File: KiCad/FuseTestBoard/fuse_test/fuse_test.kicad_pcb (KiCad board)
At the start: 2 copper layers, 20.2 x 16 mm, 1 part

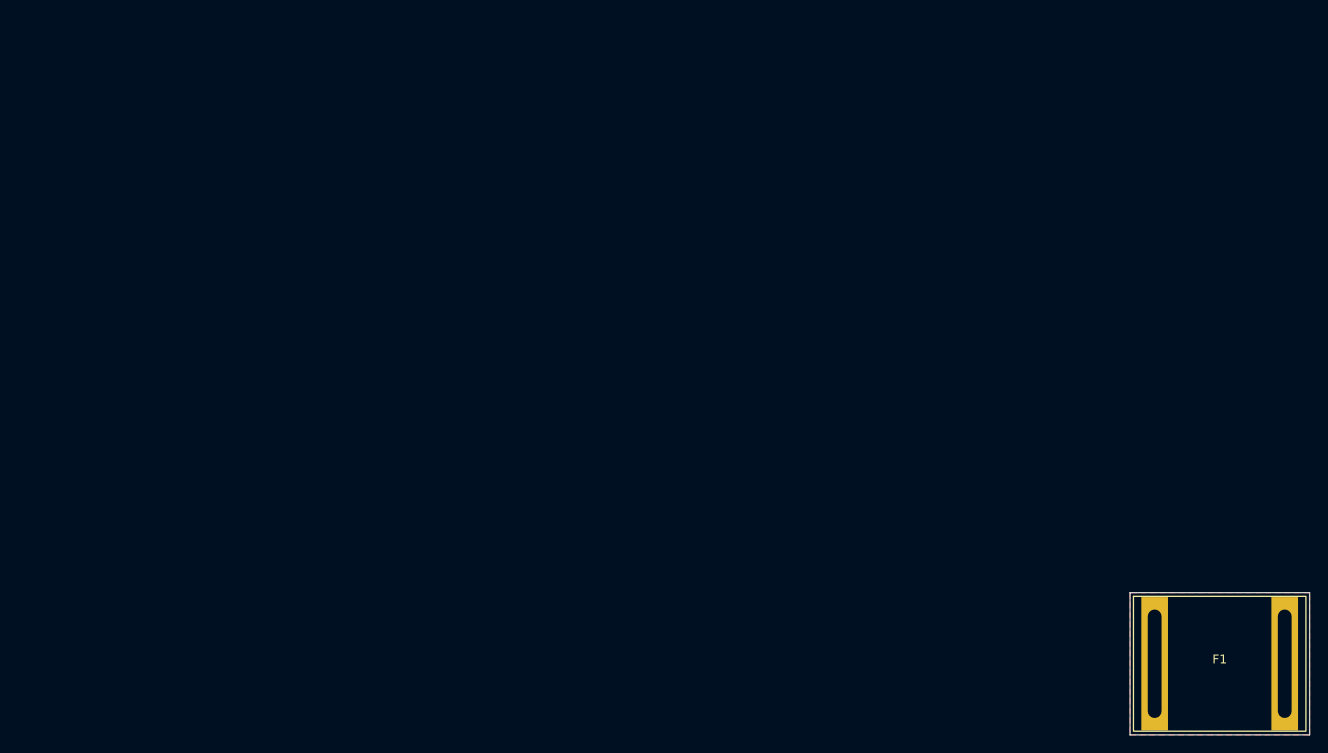
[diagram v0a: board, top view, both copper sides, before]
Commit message: adjustments to main board revision
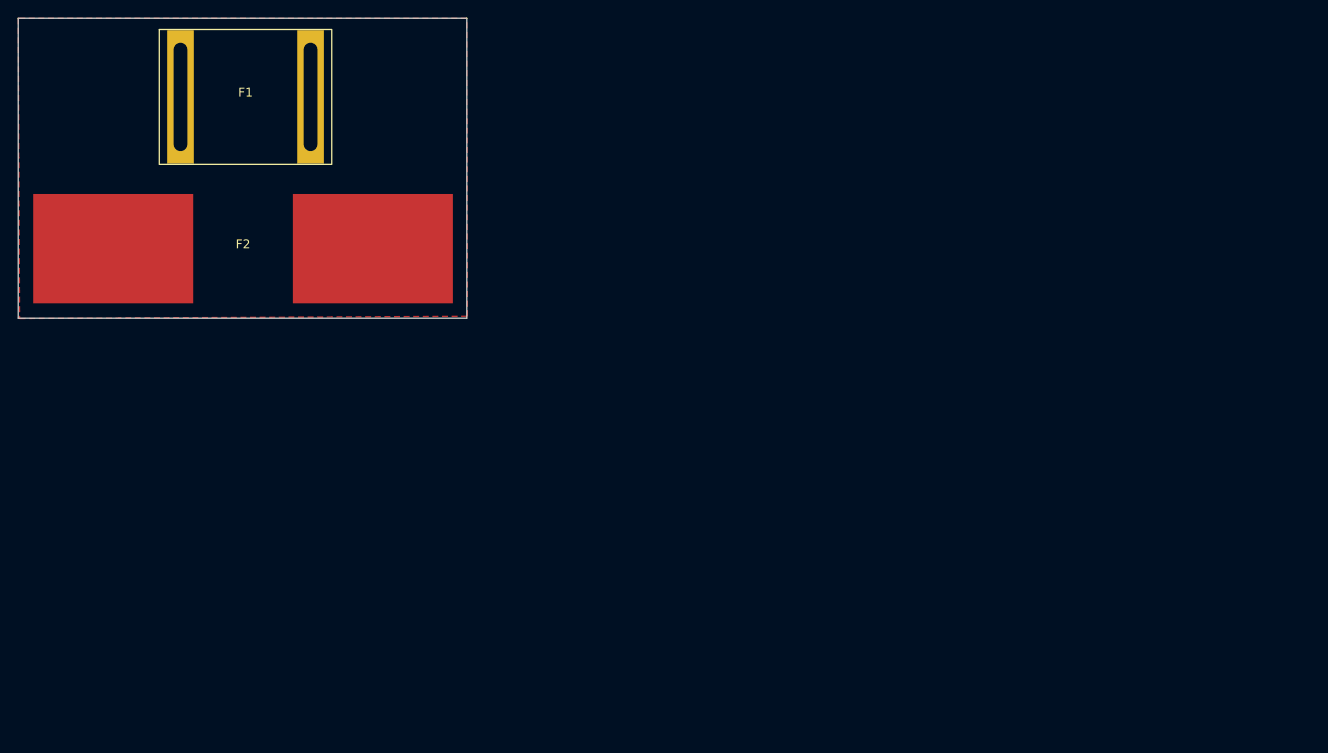
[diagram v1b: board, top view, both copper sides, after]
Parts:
- added F2: Fuse, Mechatronic Footprints:0PAL4100XP_NO_HOLES, F.Cu at (37.8, 38.3)
- F1: value 0PAL4100XP_VERTICAL -> Fuse; footprint Mechatronic Footprints:0PAL4100XP_VERTICAL -> Mechatronic Footprints:0PAL1100XP_VERTICAL
- moved F1 126.8 mm to (38.1, 21.2)
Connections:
- F1 pad 1: Net-(F1-INPUT) -> unconnected-(F1-Pad1)
- F1 pad 2: GND -> unconnected-(F1-Pad2)
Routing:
- added copper zone on F.Cu, net unconnected-(F1-Pad2)
- removed copper zone on F.Cu, net GND
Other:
- board size 20.2 x 16 mm -> 50.5 x 33.7 mm
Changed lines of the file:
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@@
   )
   (net 0 "")
-  (net 1 "Net-(F1-INPUT)")
-  (net 2 "GND")
-  (footprint "Mechatronic Footprints:0PAL4100XP_VERTICAL" (layer "F.Cu")
-    (at 147.684498 85)
+  (net 1 "unconnected-(F1-Pad1)")
+  (net 2 "unconnected-(F1-Pad2)")
+  (net 3 "unconnected-(F2-Pad1)")
+  (net 4 "unconnected-(F2-Pad2)")
+  (footprint "Mechatronic Footprints:0PAL1100XP_VERTICAL" (layer "F.Cu")
+    (at 38.1 21.2344)
     (property "Sheetfile" "fuse_test.kicad_sch")
     (property "Sheetname" "")
+    (property "ki_description" "Fuse")
+    (property "ki_keywords" "fuse")
     (attr through_hole)
     (fp_text reference "F1" (at 0 -0.5 unlocked) (layer "F.SilkS")
         (effects (font (size 1 1) (thickness 0.1)))
     )
-    (fp_text value "0PAL4100XP_VERTICAL" (at 0 -2.54 unlocked) (layer "F.Fab")
+    (fp_text value "Fuse" (at 0 -2.54 unlocked) (layer "F.Fab")
         (effects (font (size 1 1) (thickness 0.15)))
     )
@@
       (stroke (width 0.1) (type default)) (fill none) (layer "F.SilkS"))
     (pad "1" thru_hole rect (at -7.315502 0) (size 3 15) (drill oval 1.55 12.2) (layers "*.Cu" "*.Mask")
-      (net 1 "Net-(F1-INPUT)") (pinfunction "INPUT") (pintype "bidirectional"))
+      (net 1 "unconnected-(F1-Pad1)") (pintype "passive"))
     (pad "2" thru_hole rect (at 7.315502 0) (size 3 15) (drill oval 1.55 12.2) (layers "*.Cu" "*.Mask")
-      (net 2 "GND") (pinfunction "OUTPUT") (pintype "bidirectional"))
+      (net 2 "unconnected-(F1-Pad2)") (pintype "passive"))
   )
-  (gr_rect (start 137.6 77) (end 157.8 93)
+  (footprint "Mechatronic Footprints:0PAL4100XP_NO_HOLES" (layer "F.Cu")
+    (at 37.8206 38.3032)
+    (property "Sheetfile" "fuse_test.kicad_sch")
+    (property "Sheetname" "")
+    (property "ki_description" "Fuse")
+    (property "ki_keywords" "fuse")
+    (attr smd)
+    (fp_text reference "F2" (at 0 -0.5 unlocked) (layer "F.SilkS")
+        (effects (font (size 1 1) (thickness 0.15)))
+    )
+    (fp_text value "Fuse" (at 0.381 -7.874 unlocked) (layer "F.Fab")
+        (effects (font (size 1 1) (thickness 0.15)))
+    )
+    (fp_text user "${REFERENCE}" (at 0.127 2.413 unlocked) (layer "F.Fab")
+        (effects (font (size 1 1) (thickness 0.15)))
+    )
+    (pad "1" smd rect (at -14.605 0) (size 18 12.3) (layers "F.Cu" "F.Paste" "F.Mask")
+      (net 3 "unconnected-(F2-Pad1)") (pintype "passive") (thermal_bridge_angle 45))
+    (pad "2" smd rect (at 14.605 0) (size 18 12.3) (layers "F.Cu" "F.Paste" "F.Mask")
+      (net 4 "unconnected-(F2-Pad2)") (pintype "passive") (thermal_bridge_angle 45))
+  )
+  (gr_rect (start 12.530702 12.3824) (end 62.992 46.1264)
     (stroke (width 0.1) (type default)) (fill none) (layer "Edge.Cuts"))
-  (zone (net 2) (net_name "GND") (layer "F.Cu") (hatch edge 0.5)
+  (zone (net 2) (net_name "unconnected-(F1-Pad2)") (layer "F.Cu") (hatch edge 0.5)
     (connect_pads (clearance 0.5))
     (min_thickness 0.25) (filled_areas_thickness no)
@@
     (polygon
       (pts
-        (xy 137.6 77)
-        (xy 137.6 93)
-        (xy 157.8 93)
-        (xy 157.8 77)
+        (xy 12.530702 12.3824)
+        (xy 12.683102 46.1624)
+        (xy 63.058302 45.9084)
+        (xy 62.992 12.3952)
       )
     )
